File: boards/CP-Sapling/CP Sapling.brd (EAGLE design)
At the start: 28.6 x 18.5 mm, 17 parts, among them J1 1981568-1, J4 QWIIC_RIGHT_ANGLE, U1 ATSAMD21E18A-AUTTQFP32_MC_MCH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, U2 TLV75533PDBVRDBV5_TEX-L, U3 AT25DF081A-SSH-T

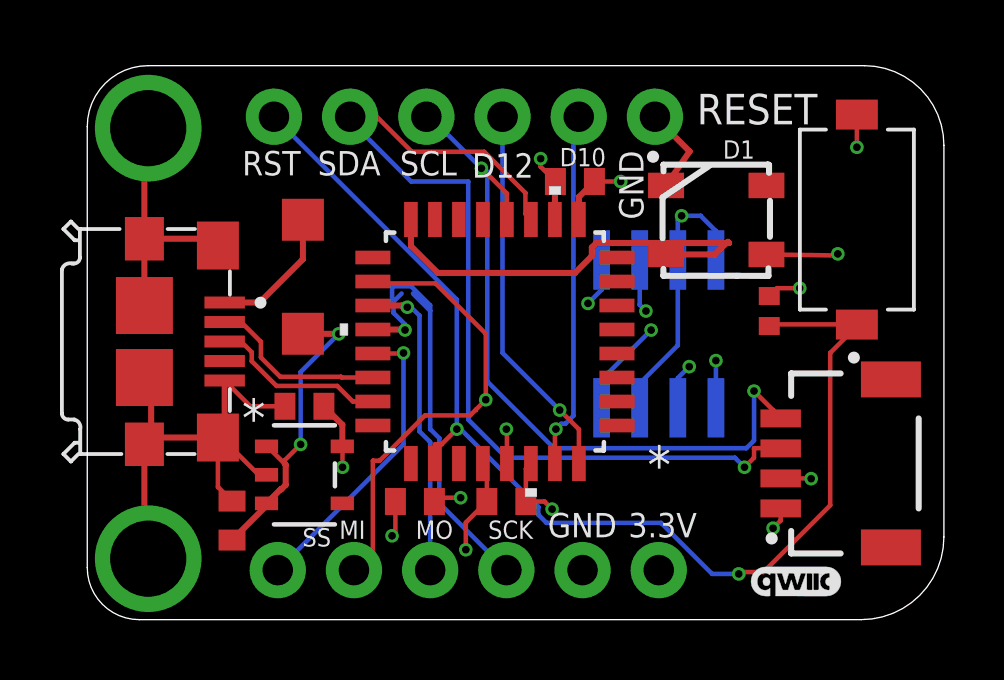
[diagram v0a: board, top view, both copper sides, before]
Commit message: Add files via upload
updating board and schematic files
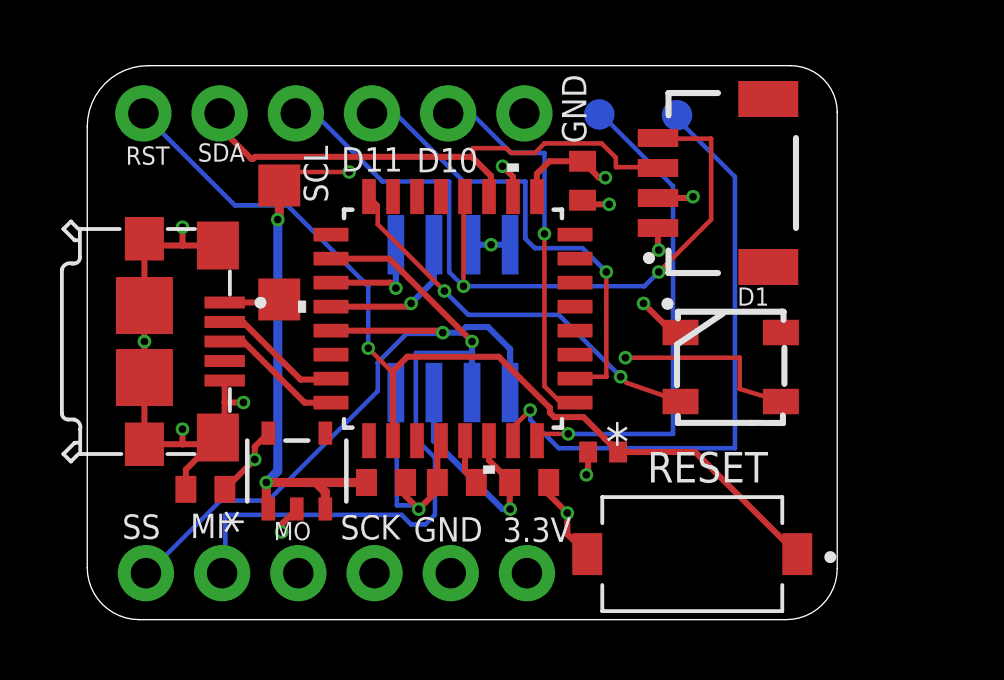
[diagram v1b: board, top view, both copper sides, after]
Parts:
- removed LOGO1: QWIIC_LOGO_3MM, SparkFun-Aesthetics:QWIIC_3MM
- added TP1, TP2: TEST-POINT3X4, SparkFun-Connectors:PAD.03X.04
- moved S1 12.4 mm to (20.2, 2.18), turned to 180 degrees
- moved J4 10.2 mm to (19.0, 14.6)
- moved R1 7.26 mm to (17.2, 5.59), turned to 180 degrees
- moved U3 6.88 mm to (12.2, 10.0)
- moved C2 5.29 mm to (9.96, 4.57), turned to 0 degrees
- moved D1 4.93 mm to (22.2, 7.67)
- moved J2 4.40 mm to (1.96, 1.55)
- moved J3 4.35 mm to (14.6, 16.9)
- moved C1 4.31 mm to (3.94, 4.34)
- moved U1 1.59 mm to (12.2, 10.0)
- moved C3 1.53 mm to (12.3, 4.57)
- moved U$1 1.45 mm to (6.35, 12.6), turned to 270 degrees
- moved C5 0.99 mm to (14.7, 4.57), turned to 0 degrees
- moved U2 0.28 mm to (6.99, 4.95), turned to 90 degrees
- moved C4 0.26 mm to (16.5, 14.6), turned to 270 degrees
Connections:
- net D1 renamed NP
- removed net SWCLK/D10: J3.2, U1.31
- removed net SWDIO/D12: J3.3, U1.32
- new net D10: J3.2, U1.1
- new net D11: J3.3, U1.2
- new net SWCLK: TP2.P$1, U1.31
- new net SWDIO: TP1.P$1, U1.32
- net DM: now also U1.23; no longer U1.22
- net DP: now also U1.24; no longer U1.23
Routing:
- net SWCLK: track 0.00 -> 20.7 mm, vias 0 -> 1
- net SWDIO: track 0.00 -> 16.4 mm, vias 0 -> 1
- net D11: track 0.00 -> 15.7 mm, vias 0 -> 1
- net SDA: track 32.2 -> 18.2 mm, vias 1 -> 0
- net D10: track 0.00 -> 12.8 mm, vias 0 -> 1
- net SWDIO/D12: track 12.6 -> 0.00 mm, vias 1 -> 0
- net SWCLK/D10: track 12.0 -> 0.00 mm, vias 1 -> 0
- net SCK: track 25.6 -> 14.5 mm, vias 2 -> 1
- net RESET: track 39.4 -> 31.9 mm, vias 2 -> 1
- net VUSB: track 30.6 -> 35.9 mm, vias 3 -> 4
- net MOSI: track 18.0 -> 14.6 mm, vias 2 -> 1
- net N$4: track 5.00 -> 1.55 mm, vias 2 -> 0
- net GND: track 40.6 -> 37.5 mm, vias 8 -> 11
- net N$1: track 4.52 -> 1.86 mm
- net SCL: track 24.7 -> 26.4 mm
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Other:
- board size 28.6 x 18.5 mm -> 25 x 18.5 mm
- board text added: "D1"
- board text added: "D11"
- board text added: "SWCLK"
- board text added: "SWDIO"
- board text removed: "D12"
